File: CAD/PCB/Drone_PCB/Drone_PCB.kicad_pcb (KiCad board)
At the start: 2 copper layers, 28 parts, among them J1 MEM2051-00-195-00-A, J3 10118193-0001LF, SW1 PTS 647 SN50 SMTR2 LFS, U1 RP2040, U2 NCP1117-3.3_SOT223, U3 ICM-20948, U5 W25Q128JVSIQ TR, Y1 ABLS-12.000MHZ-K2-T

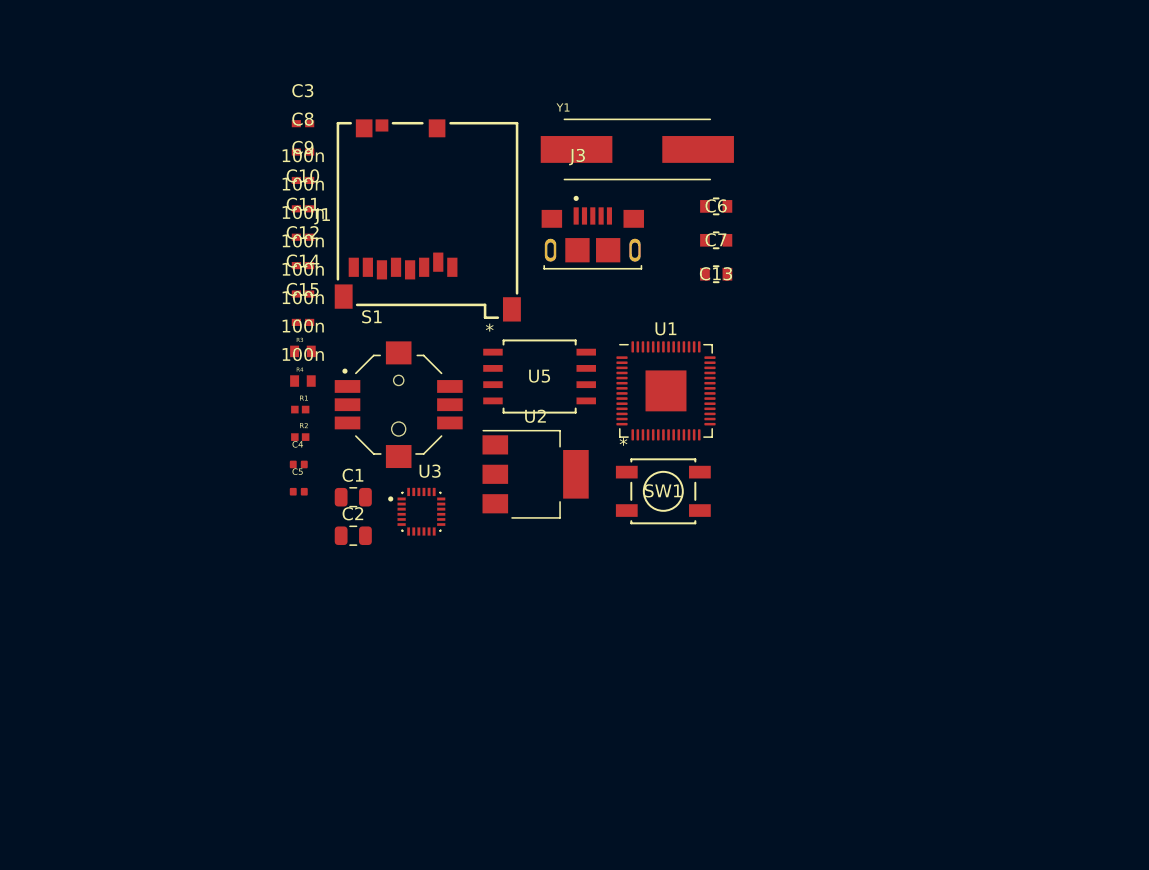
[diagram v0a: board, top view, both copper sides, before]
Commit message: stuff
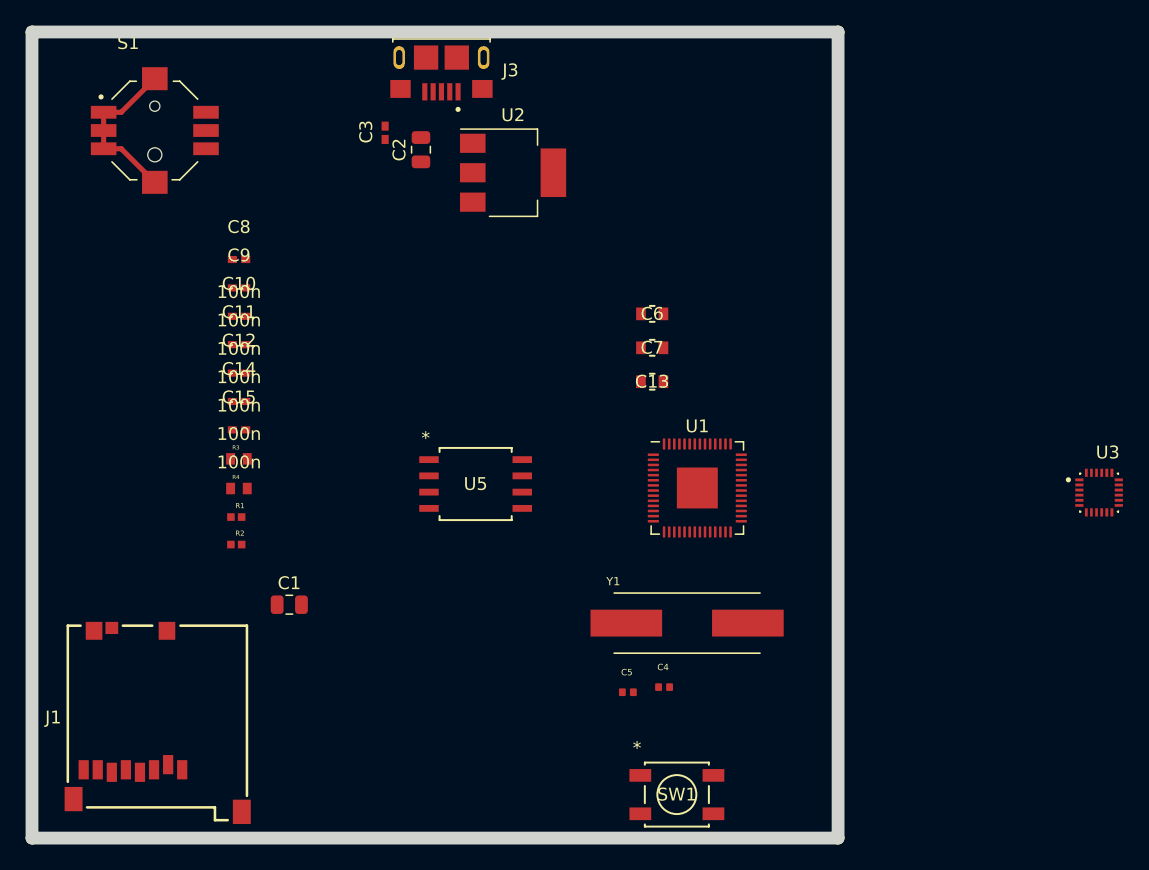
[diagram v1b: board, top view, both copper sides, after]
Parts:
- moved U3 53.0 mm to (201.6, 100.0)
- moved J1 44.6 mm to (128.0, 118.0)
- moved Y1 37.2 mm to (169.4, 110.2)
- moved C4 33.4 mm to (167.6, 115.2)
- moved C2 30.6 mm to (148.6, 73.2), turned to 90 degrees
- moved C5 30.1 mm to (164.8, 115.6)
- moved S1 28.7 mm to (127.8, 71.7)
- moved SW1 23.7 mm to (168.6, 123.6)
- moved U2 23.6 mm to (155.8, 75.0)
- moved J3 19.1 mm to (150.2, 66.0), turned to 180 degrees
- moved C1 9.78 mm to (138.3, 108.8)
- moved C12 9.78 mm to (134.4, 90.7)
- moved C13 9.78 mm to (166.7, 91.3)
- moved C14 9.78 mm to (134.4, 92.9)
- moved C15 9.78 mm to (134.4, 95.1)
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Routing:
- net GND: track 0.00 -> 13.0 mm
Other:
- board outline added: 63 x 63 mm
